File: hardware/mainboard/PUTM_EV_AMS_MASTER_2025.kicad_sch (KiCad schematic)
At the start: 36 parts, among them IC11 ISO6760, IC7 ISO6760, IC8 3.3V/0.5A, J1 M80-5100642, J10 M300-MV10345M1, J12 M80-51034XX, J4 FTSH-107-01-L-D-K, J5 M80-51004XX, J7 M300-MV10345M1, J8 M80-51004XX, U4 UCC12040DVE

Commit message: schematic?
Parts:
- removed C39, C44, C45, C46, C47, C48: 100nF, Capacitor_SMD:C_0603_1608Metric, symbol Device:C_Small
- removed C40, C59, C77: 22uF, Capacitor_SMD:C_0805_2012Metric, symbol Device:C_Small
- removed F6, F7: 5V/0.5A, Fuse:Fuse_0805_2012Metric, symbol Device:Polyfuse_Small
- removed IC11, IC7: ISO6760, Package_SO:SOIC-16W_7.5x10.3mm_P1.27mm, symbol Samacsys_kicad_sym:ISO6760
- removed IC8: 3.3V/0.5A, Package_TO_SOT_SMD:SOT-23-5, symbol AP7365-33YRG-13:AP7365-33YRG-13
- removed J12: M80-51034XX, Samacsys:M80-51034YY, symbol Samacsys_kicad_sym:M80-51034XX
- removed R22: 200, Resistor_SMD:R_0603_1608Metric, symbol Device:R_Small
- removed TP4, TP5, TP6, TP7, TP8: TestPoint_Small, TestPoint:TestPoint_THTPad_D1.0mm_Drill0.5mm, symbol Connector:TestPoint_Small
- removed U4: UCC12040DVE, Package_SO:SOIC-16W_7.5x10.3mm_P1.27mm, symbol Samacsys_kicad_sym:UCC12040DVE
- added C81: 100pF, Capacitor_SMD:C_0603_1608Metric, symbol Device:C_Small
- added D21, D22: 3.6V/400W, Package_TO_SOT_SMD:SOT-23-6, symbol Power_Protection:ESDA5V3SC5
- added D23: 5.3V/400W, Package_TO_SOT_SMD:SOT-23-3, symbol Power_Protection:ESDA5V3L
- added J2: M80-5102042, Samacsys:M80-51020YY, symbol Samacsys_kicad_sym:M80-5102042
- added J3: M80-5100842, Samacsys:M80-51008YY, symbol Samacsys_kicad_sym:M80-5100842
- added T1: SM91502ALE, Samacsys:SOP254P927X572-6N, symbol Samacsys_kicad_sym:SM91502ALE
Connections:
- net GNDISO is gone; now on net GND: J8.4 (Pin_4)
- net AIR_M_DETECTION: now also J2.15
- net AIR_PRE_DETECTION: now also J2.14
- net AIR_P_DETECTION: now also J2.13
- net CANFD1+: now also J2.3
- net CANFD1-: now also J2.4
- net CANFD2+: now also J2.5
- net CANFD2-: now also J2.6
- net CAR_I: now also D23.1 (K)
- net CCO+: now also T1.3 (PRI_3)
- net CCO-: now also T1.1 (PRI_1)
- net CHARGER_DETECTION: now also J2.12
- net FAN1-: now also J3.1
- net FAN2-: now also J3.2
- net FAN3-: now also J3.3
- net FAN4-: now also J3.4
- net GND: now also C81.2, D21.2 (K), D21.5 (NC), D22.2 (K), D22.5 (NC), D23.3 (A), J2.11, J2.19, J2.20
- net NRST: now also D21.4 (A)
- net SAFETY_IN: now also J2.8
- net SAFETY_OUT: now also J2.7
- net SWCLK: now also D21.3 (A)
- net SWDIO: now also D21.1 (A)
- net TSMS: now also J2.18
- net UART_RX: now also D22.1 (A)
- net UART_TX: now also D21.6 (A)
- net VDD: now also J2.10
- net +3.3V renamed +3.3VIO
- net +3.3VIO: now also D22.3 (A)
- net +5VISO: no longer names the net of J8.3 (Pin_3)
- net ACU+ renamed IsolationBarrier/ACU_IN+
- net ACU- renamed IsolationBarrier/ACU_IN-
- net CAR+ renamed IsolationBarrier/CAR_IN+
- net CAR- renamed IsolationBarrier/CAR_IN-
- net CAR_I_REF renamed +5VA
- net +5VA: now also D23.2 (K)
- new net: C81.1, T1.5 (SEC_2)
- new net +24V: J3.5, J3.6, J3.7, J3.8
- new net +8V: J2.9
- new net D+: J2.2
- new net D-: J2.1
- new net Isolated SPI/OUT+: T1.4 (SEC_1)
- new net Isolated SPI/OUT-: T1.6 (SEC_3)
- new net VBUS+: J2.17
- no-connect marks 26 -> 12
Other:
- sheet Isolated ADC renamed ADC
- added sheet IsolationBarrier (IsolationBarrier.kicad_sch)
- sheet ADC: file IsolatedADC.kicad_sch -> ADC.kicad_sch
- sheet ADC ports: added none; removed CAR_I_REF
- sheet Connectivity ports: added EX_D+, EX_D-, FTDI_RX, FTDI_TX; removed EX_USB_D+, EX_USB_D-, UC_D+, UC_D-
- sheet Isolated SPI ports: added RX, TX; removed MISO, MOSI, SCK, SPI_RDY, ~{CS}
- sheet MCU ports: added DETECT_USB, SIGNAL_LED_ERR, SIGNAL_LED_OK, SIGNAL_LED_WRN, UART_COM_RX, UART_COM_TX, UART_DEBUG_RX, UART_DEBUG_TX, UART_USB_RX, UART_USB_TX; removed COM_MISO, D+, D-, SIGNAL_LED_1, SIGNAL_LED_2, SIGNAL_LED_3, SPI_RDY, UART_RX, UART_TX
- sheet Power ports: added VBUS_SENSE; removed none
- sheet Safety ports: added none; removed DASH_LED_ERROR
- note added: "ADC"
- note added: "AIR"
- note added: "COM"
- note added: "CURRENT"
- note added: "FAN"
- note added: "USBGND"
- note removed: "ADC AND SPI"
- note removed: "AIR CONNECTORS"
- note removed: "AIR CONTROL"
- note removed: "CONNECTORS"
- note removed: "FAN CONNECTORS"
- note removed: "FAN CONTROL"
- note removed: "GALVANIC ISOLATION"
- note removed: "ISO POWER"
- note removed: "SHARED"
- note removed: "TI_IC ONLY"
- moved on the sheet: D1, D2, D3, D6, J1, J10, J4, J5, J7, J8, R27, R31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

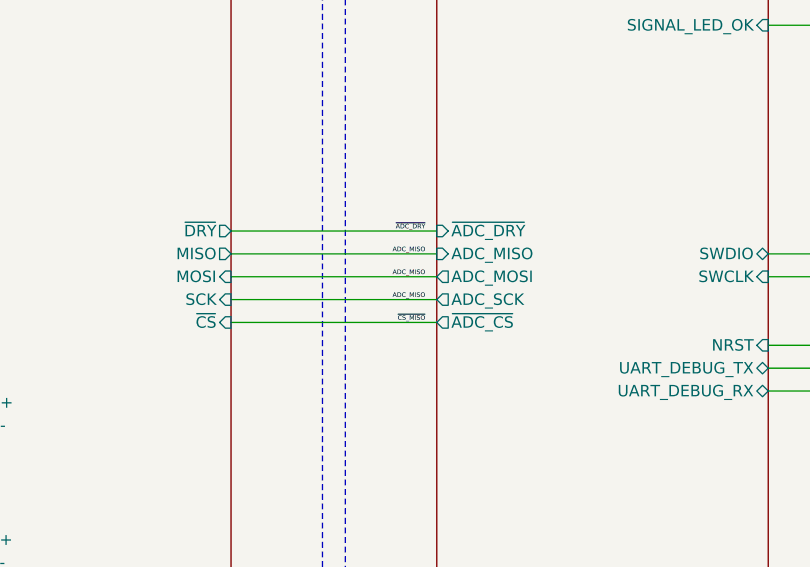
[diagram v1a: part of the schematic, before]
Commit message: sync
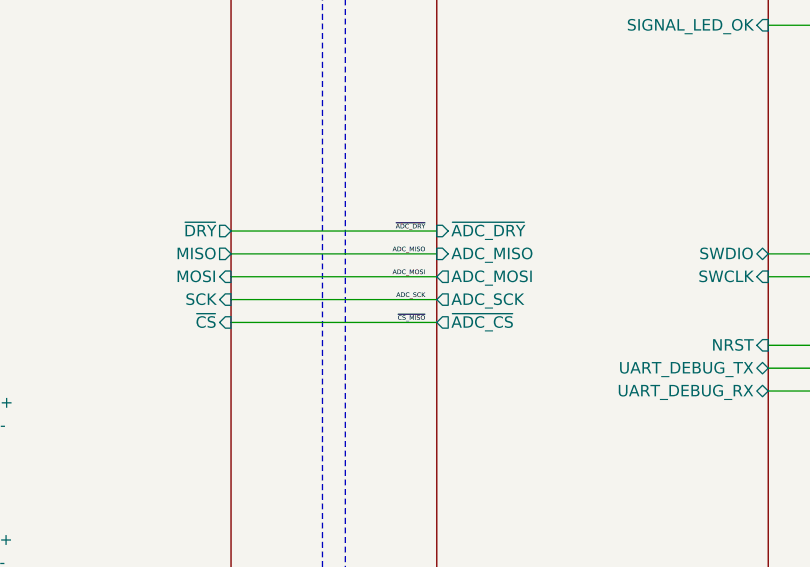
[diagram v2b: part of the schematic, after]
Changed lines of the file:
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@@
+		)
+	)
+	(label "ADC_MOSI"
+		(at 182.88 81.28 180)
+		(effects
+			(font
+				(size 0.508 0.508)
+			)
+			(justify right bottom)
 		)
 	)
@@
 	)
 	(label "ADC_MISO"
-		(at 182.88 81.28 180)
+		(at 182.88 78.74 180)
 		(effects
 			(font
@@
 		)
 	)
+	(label "ADC_SCK"
+		(at 182.88 83.82 180)
+		(effects
+			(font
+				(size 0.508 0.508)
+			)
+			(justify right bottom)
+		)
+	)
 	(label "FC1"
 		(at 182.88 259.08 180)
@@
 		)
 	)
-	(label "ADC_MISO"
-		(at 182.88 78.74 180)
-		(effects
-			(font
-				(size 0.508 0.508)
-			)
-			(justify right bottom)
-		)
-	)
 	(label "CTX1"
 		(at 222.25 187.96 0)
@@
 		)
 	)
-	(label "ADC_MISO"
-		(at 182.88 83.82 180)
-		(effects
-			(font
-				(size 0.508 0.508)
-			)
-			(justify right bottom)
-		)
-	)
 	(label "NRST"
 		(at 335.28 88.9 180)
@@
 		)
 	)
+	(netclass_flag ""
+		(length 2.54)
+		(shape round)
+		(at 75.2666 149.86 0)
+		(fields_autoplaced yes)
+		(effects
+			(font
+				(size 1.27 1.27)
+			)
+			(justify left bottom)
+		)
+		(property "Netclass" "120Ohm"
+			(at 74.657 147.32 0)
+			(effects
+				(font
+					(size 1.27 1.27)
+				)
+				(justify right)
+			)
+		)
+		(property "Component Class" ""
+			(at 348.3166 57.15 0)
+			(effects
+				(font
+					(size 1.27 1.27)
+					(italic yes)
+				)
+				(justify left)
+			)
+		)
+	)
+	(netclass_flag ""
+		(length 2.54)
+		(shape round)
+		(at 75.2666 152.4 180)
+		(fields_autoplaced yes)
+		(effects
+			(font
+				(size 1.27 1.27)
+			)
+			(justify right bottom)
+		)
+		(property "Netclass" "120Ohm"
+			(at 74.657 154.94 0)
+			(effects
+				(font
+					(size 1.27 1.27)
+				)
+				(justify right)
+			)
+		)
+		(property "Component Class" ""
+			(at 348.3166 245.11 0)
+			(effects
+				(font
+					(size 1.27 1.27)
+					(italic yes)
+				)
+				(justify left)
+			)
+		)
+	)

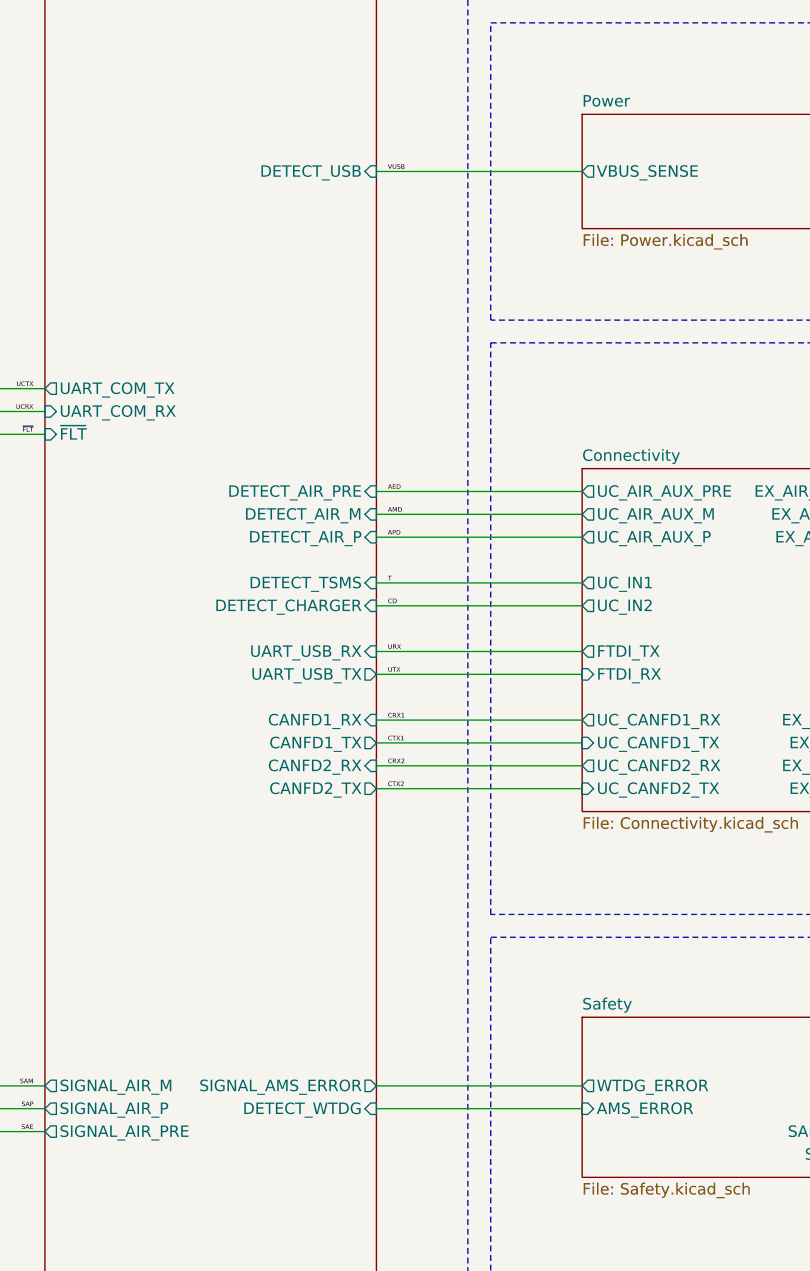
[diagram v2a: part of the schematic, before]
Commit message: sync
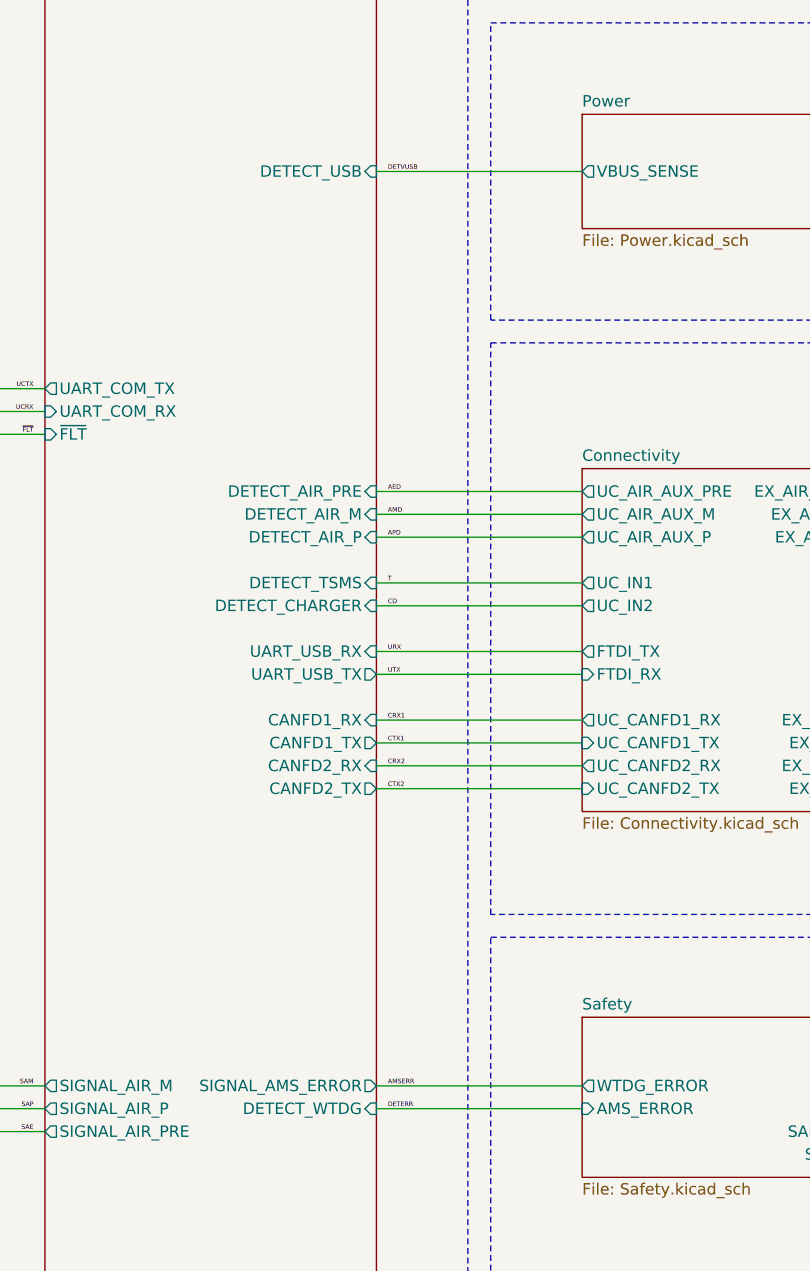
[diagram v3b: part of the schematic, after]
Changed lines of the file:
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@@
+		)
+	)
+	(label "AMSERR"
+		(at 222.25 226.06 0)
+		(effects
+			(font
+				(size 0.508 0.508)
+			)
+			(justify left bottom)
 		)
 	)
@@
 		)
 	)
-	(label "VUSB"
+	(label "DETVUSB"
 		(at 222.25 124.46 0)
 		(effects
 			(font
+				(size 0.508 0.508)
+			)
+			(justify left bottom)
+		)
+	)
+	(label "DETERR"
+		(at 222.25 228.6 0)
+		(effects
+			(font

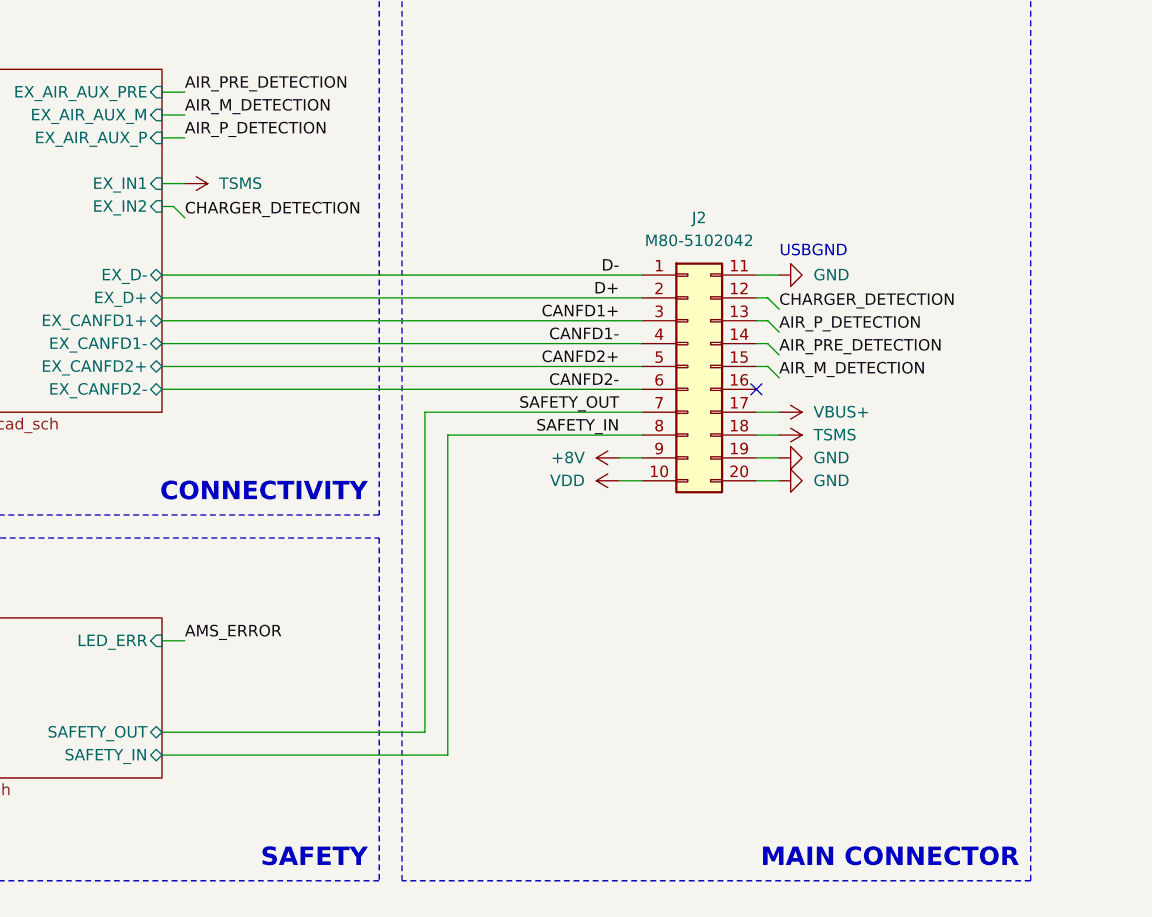
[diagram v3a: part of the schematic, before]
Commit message: sync
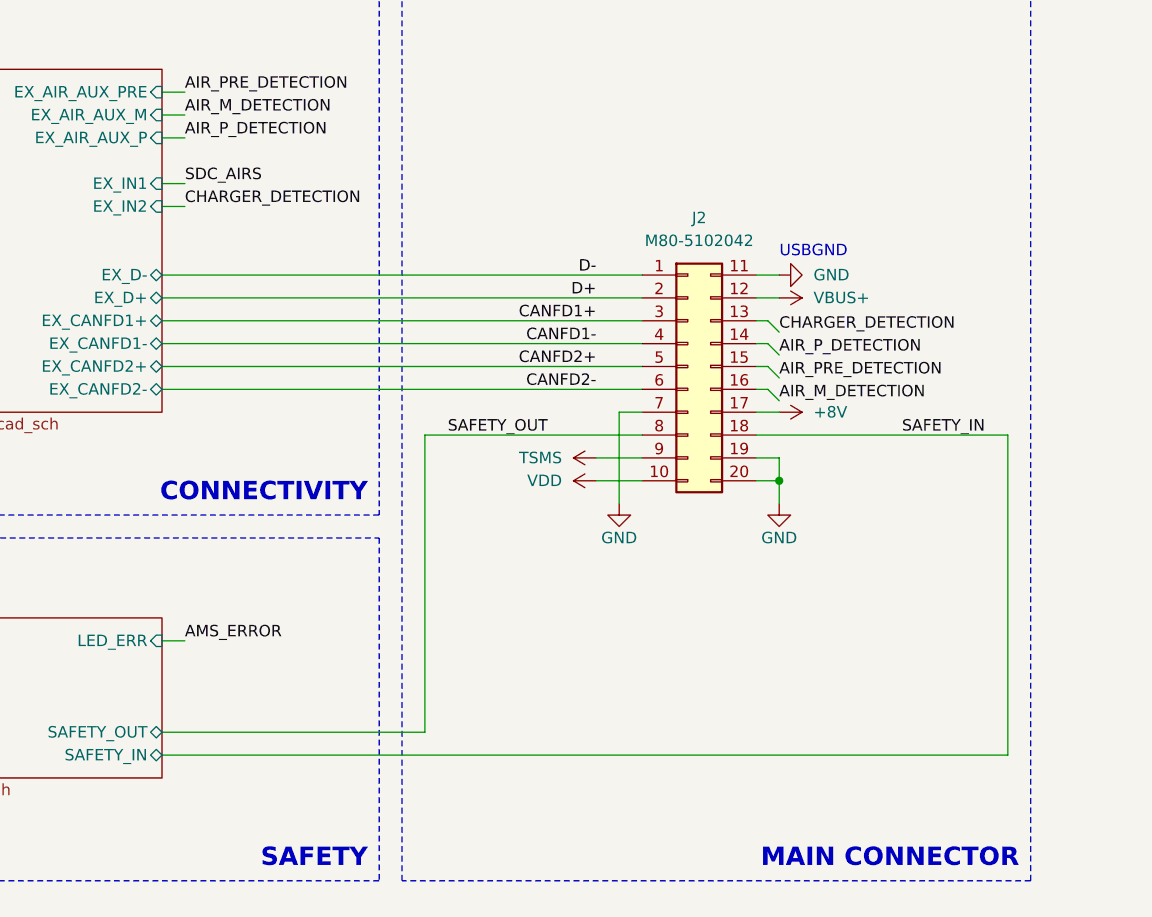
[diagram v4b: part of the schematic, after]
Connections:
- net +8V: now also J2.17; no longer J2.9
- net AIR_M_DETECTION: now also J2.16; no longer J2.15
- net AIR_PRE_DETECTION: now also J2.15; no longer J2.14
- net AIR_P_DETECTION: now also J2.14; no longer J2.13
- net CHARGER_DETECTION: now also J2.13; no longer J2.12
- net GND: now also J2.7
- net SAFETY_IN: now also J2.18; no longer J2.8
- net SAFETY_OUT: now also J2.8; no longer J2.7
- net TSMS: now also J2.9; no longer J2.18
- net VBUS+: now also J2.12; no longer J2.17
- no-connect marks 12 -> 11
